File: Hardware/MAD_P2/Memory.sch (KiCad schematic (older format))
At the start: 5 parts, among them J5 Micro_SD_Card, U26 W25Q128JVS

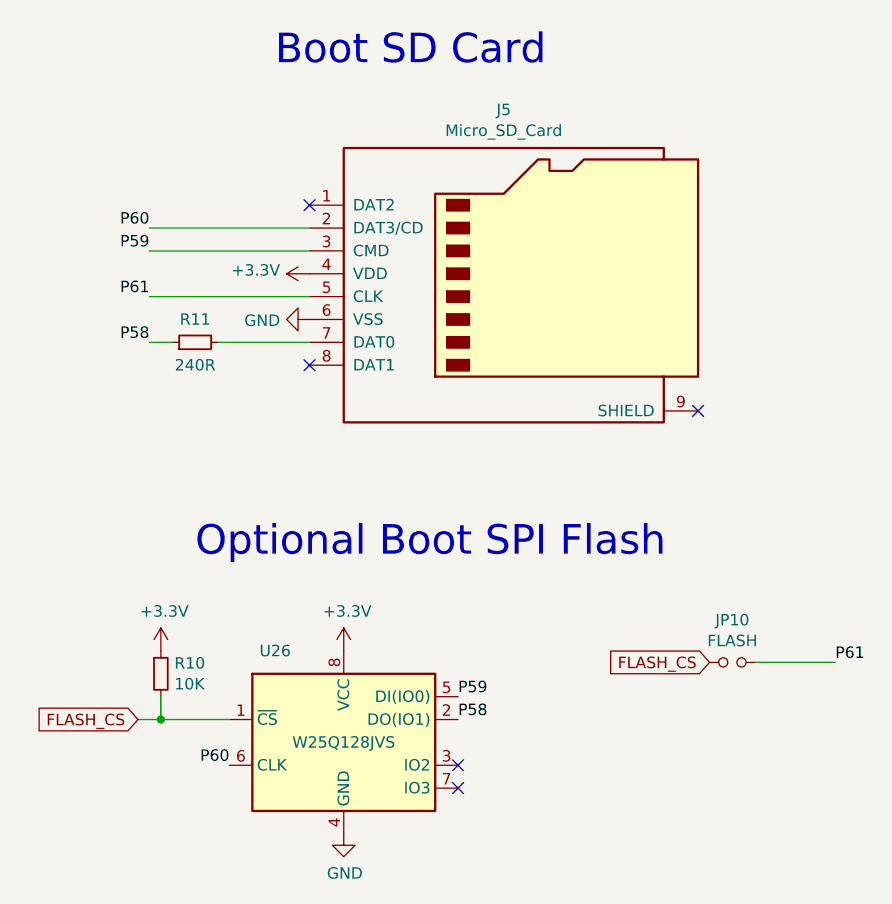
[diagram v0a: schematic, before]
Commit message: revising pcb layout
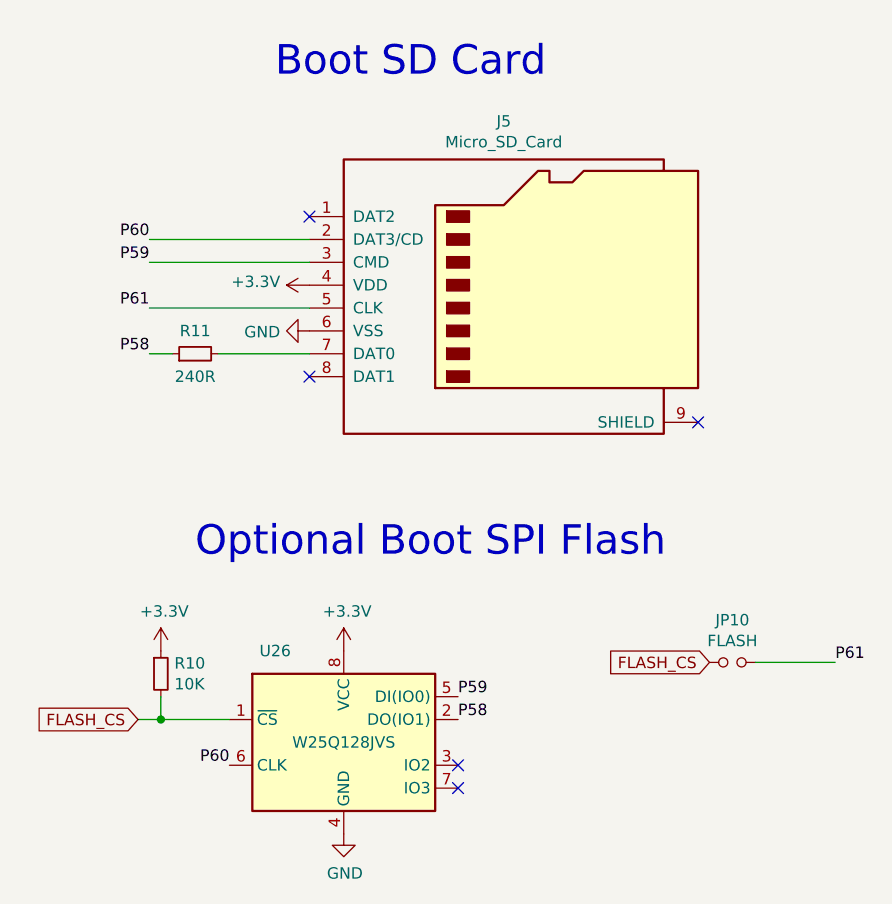
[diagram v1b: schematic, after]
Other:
- moved on the sheet: J5, R11
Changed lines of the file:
@@
 L Connector:Micro_SD_Card J5
 U 1 1 60B0E24B
-P 6150 3300
-F 0 "J5" H 6100 4017 50  0000 C CNN
-F 1 "Micro_SD_Card" H 6100 3926 50  0000 C CNN
-F 2 "Connector_Card:microSD_HC_Hirose_DM3D-SF" H 7300 3600 50  0001 C CNN
-F 3 "http://katalog.we-online.de/em/datasheet/693072010801.pdf" H 6150 3300 50  0001 C CNN
-	1    6150 3300
+P 6150 3350
+F 0 "J5" H 6100 4067 50  0000 C CNN
+F 1 "Micro_SD_Card" H 6100 3976 50  0000 C CNN
+F 2 "Connector_Card:microSD_HC_Hirose_DM3D-SF" H 7300 3650 50  0001 C CNN
+F 3 "http://katalog.we-online.de/em/datasheet/693072010801.pdf" H 6150 3350 50  0001 C CNN
+	1    6150 3350
 	1    0    0    -1
 $EndComp
@@
 L power:+3.3V #PWR0142
 U 1 1 60B14DB5
-P 5250 3300
-F 0 "#PWR0142" H 5250 3150 50  0001 C CNN
-F 1 "+3.3V" V 5265 3428 50  0000 L CNN
-F 2 "" H 5250 3300 50  0001 C CNN
-F 3 "" H 5250 3300 50  0001 C CNN
-	1    5250 3300
+P 5250 3350
+F 0 "#PWR0142" H 5250 3200 50  0001 C CNN
+F 1 "+3.3V" V 5265 3478 50  0000 L CNN
+F 2 "" H 5250 3350 50  0001 C CNN
+F 3 "" H 5250 3350 50  0001 C CNN
+	1    5250 3350
 	0    -1   -1   0
 $EndComp
@@
 L power:GND #PWR0143
 U 1 1 60B15F33
-P 5250 3500
-F 0 "#PWR0143" H 5250 3250 50  0001 C CNN
-F 1 "GND" V 5255 3372 50  0000 R CNN
-F 2 "" H 5250 3500 50  0001 C CNN
-F 3 "" H 5250 3500 50  0001 C CNN
-	1    5250 3500
+P 5250 3550
+F 0 "#PWR0143" H 5250 3300 50  0001 C CNN
+F 1 "GND" V 5255 3422 50  0000 R CNN
+F 2 "" H 5250 3550 50  0001 C CNN
+F 3 "" H 5250 3550 50  0001 C CNN
+	1    5250 3550
 	0    1    1    0
 $EndComp
-NoConn ~ 6950 3900
-Text Label 4550 3100 2    50   ~ 0
+NoConn ~ 6950 3950
+Text Label 4550 3150 2    50   ~ 0
 P60
-Text Label 4550 3200 2    50   ~ 0
+Text Label 4550 3250 2    50   ~ 0
 P59
-Text Label 4550 3400 2    50   ~ 0
+Text Label 4550 3450 2    50   ~ 0
 P61
-Text Label 4550 3600 2    50   ~ 0
+Text Label 4550 3650 2    50   ~ 0
 P58
-NoConn ~ 5250 3700
-NoConn ~ 5250 3000
+NoConn ~ 5250 3750
+NoConn ~ 5250 3050
 $Comp
 L Device:R_Small R11
 U 1 1 60B28350
-P 4750 3600
-F 0 "R11" V 4850 3600 50  0000 C CNN
-F 1 "240R" V 4650 3600 50  0000 C CNN
-F 2 "Resistor_SMD:R_0603_1608Metric" H 4750 3600 50  0001 C CNN
-F 3 "~" H 4750 3600 50  0001 C CNN
-	1    4750 3600
+P 4750 3650
+F 0 "R11" V 4850 3650 50  0000 C CNN
+F 1 "240R" V 4650 3650 50  0000 C CNN
+F 2 "Resistor_SMD:R_0603_1608Metric" H 4750 3650 50  0001 C CNN
+F 3 "~" H 4750 3650 50  0001 C CNN
+	1    4750 3650
 	0    -1   -1   0
 $EndComp
@@
 	7550 5000 7200 5000
 Wire Wire Line
-	4550 3600 4650 3600
+	4550 3650 4650 3650
 Wire Wire Line
-	4850 3600 5250 3600
+	4850 3650 5250 3650
 Wire Wire Line
-	4550 3400 5250 3400
+	4550 3450 5250 3450
 Wire Wire Line
-	4550 3200 5250 3200
+	4550 3250 5250 3250
 Wire Wire Line
-	4550 3100 5250 3100
+	4550 3150 5250 3150
 $Comp
 L Memory_Flash:W25Q128JVS U26
@@
 Text Notes 4750 4550 0    129  ~ 0
 Optional Boot SPI Flash
-Text Notes 5100 2400 0    129  ~ 0
+Text Notes 5100 2450 0    129  ~ 0
 Boot SD Card
 $EndSCHEMATC
